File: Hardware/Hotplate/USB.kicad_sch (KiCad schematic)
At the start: 14 parts, among them IC2 FT231XQ-T, J8 GSB1C41110SSHR

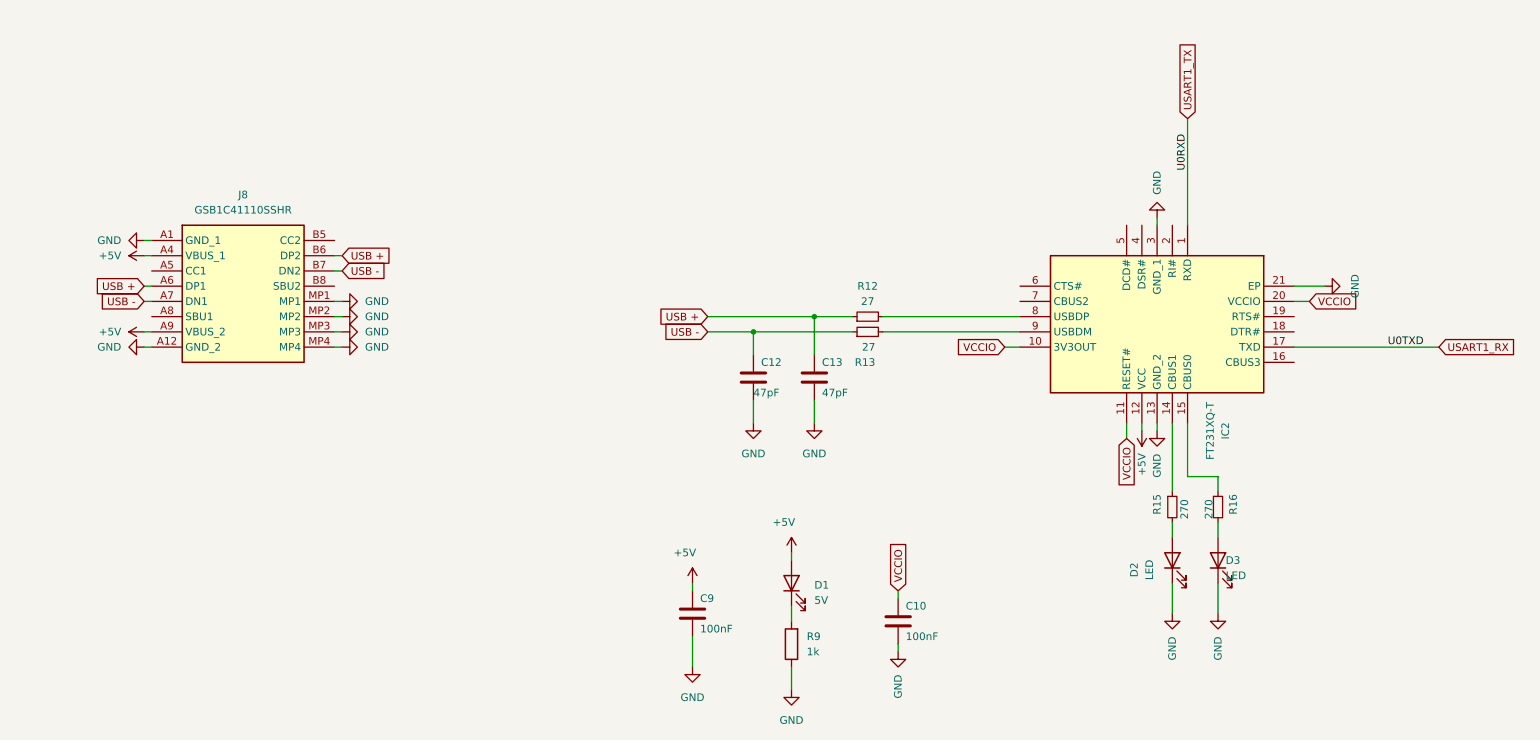
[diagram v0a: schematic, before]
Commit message: V2
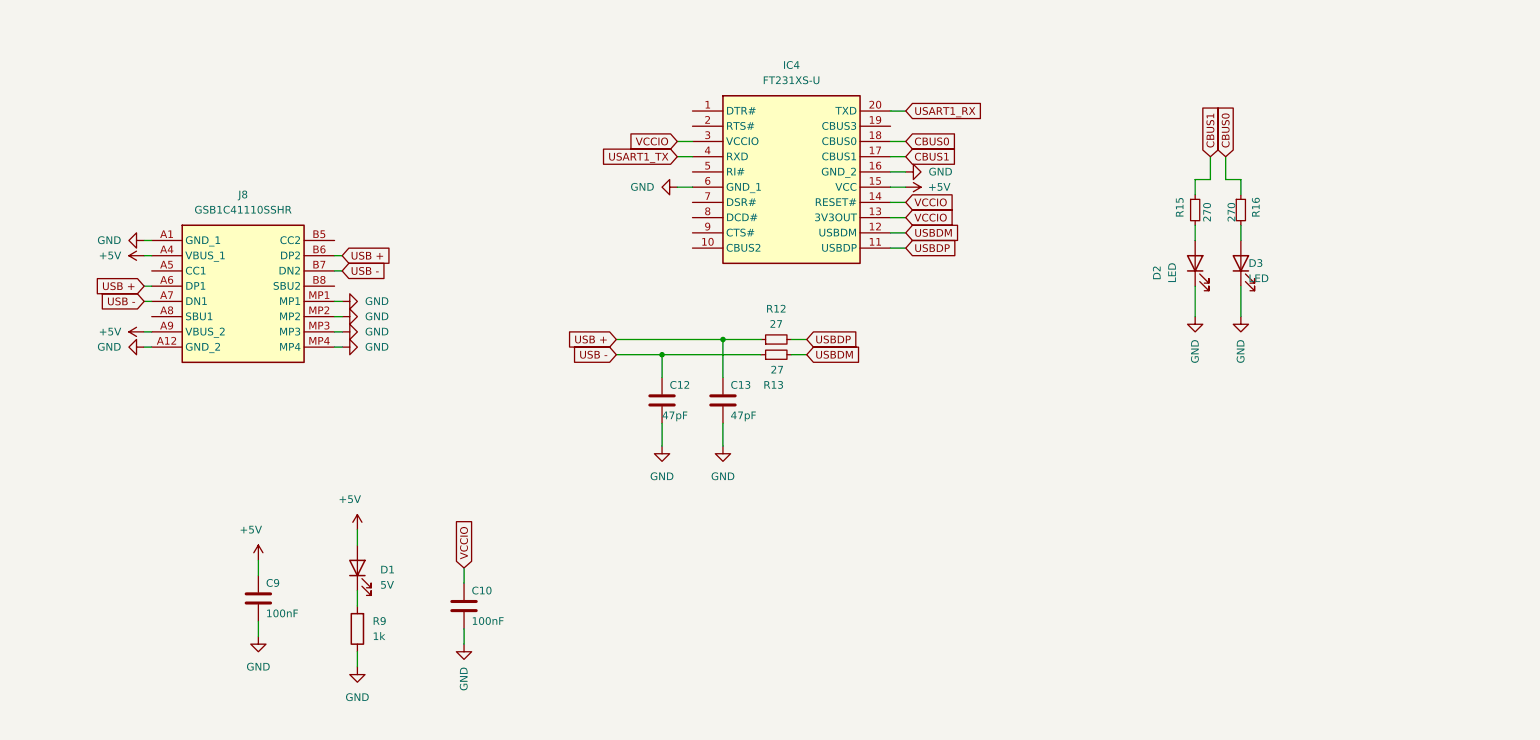
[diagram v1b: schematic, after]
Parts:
- removed IC2: FT231XQ-T, QFN50P400X400X80-21N, symbol SamacSys_Parts:FT231XQ-T
- added IC4: FT231XS-U, SOP64P599X175-20N, symbol SamacSys_Parts:FT231XS-U
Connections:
- net +5V: now also IC4.15 (VCC)
- net GND: now also IC4.16 (GND_2), IC4.6 (GND_1)
- net USART1_RX: now also IC4.20 (TXD)
- net USART1_TX: now also IC4.4 (RXD)
- net VCCIO: now also IC4.13 (3V3OUT), IC4.14 (RESET#), IC4.3 (VCCIO)
- net CBUS1: now reaches R15.1
- net CBUS1: now also IC4.17 (CBUS1)
- net CBUS0: now reaches R16.1
- net CBUS0: now also IC4.18 (CBUS0)
- net USBDM: now reaches R13.2
- net USBDM: now also IC4.12 (USBDM)
- net USBDP: now reaches R12.2
- net USBDP: now also IC4.11 (USBDP)
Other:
- moved on the sheet: C10, C12, C13, C9, D1, D2, D3, R12, R13, R15, R16, R9

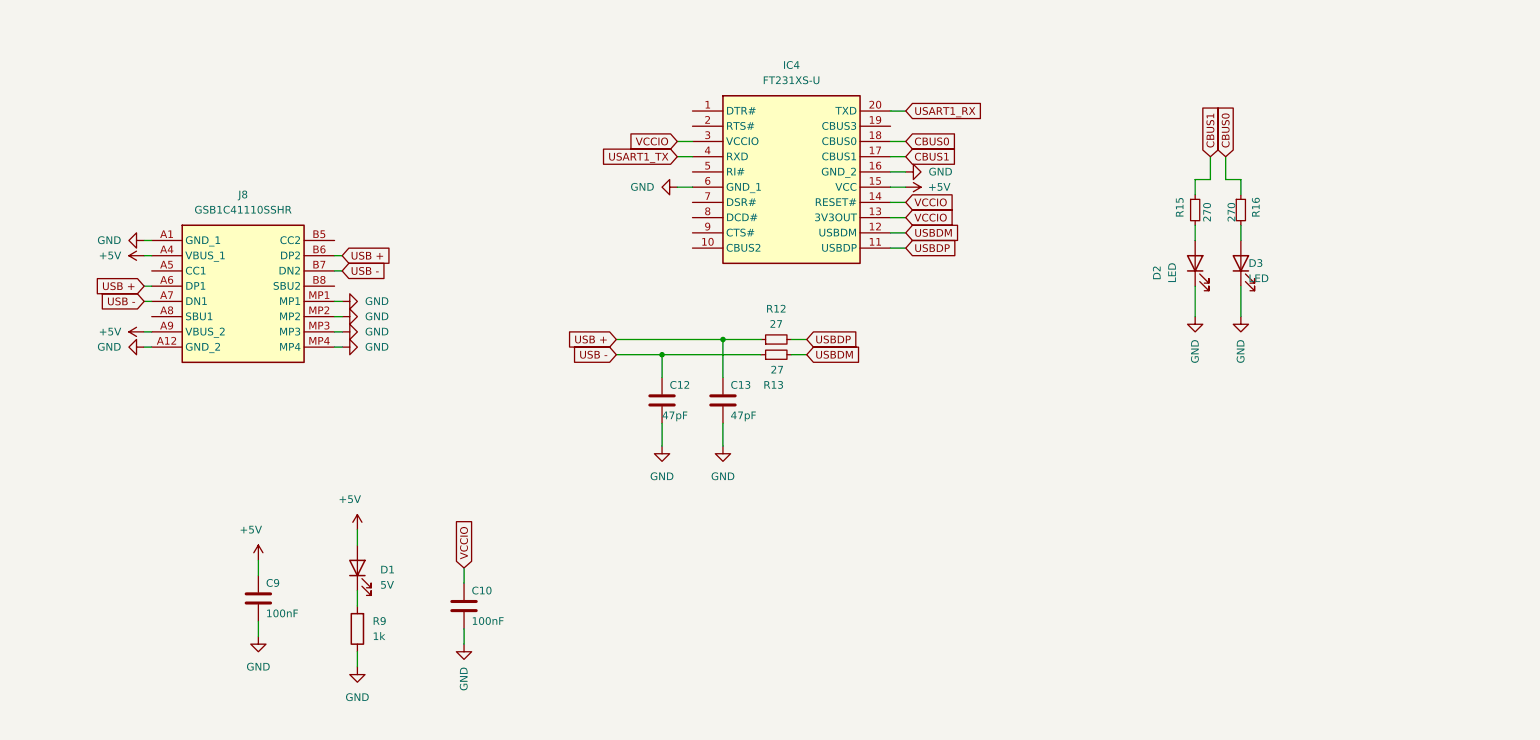
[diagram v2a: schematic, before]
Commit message: made it pretty (#8)
Co-authored-by: nexophoenixe <jan.gradwohl2005@mail.com>
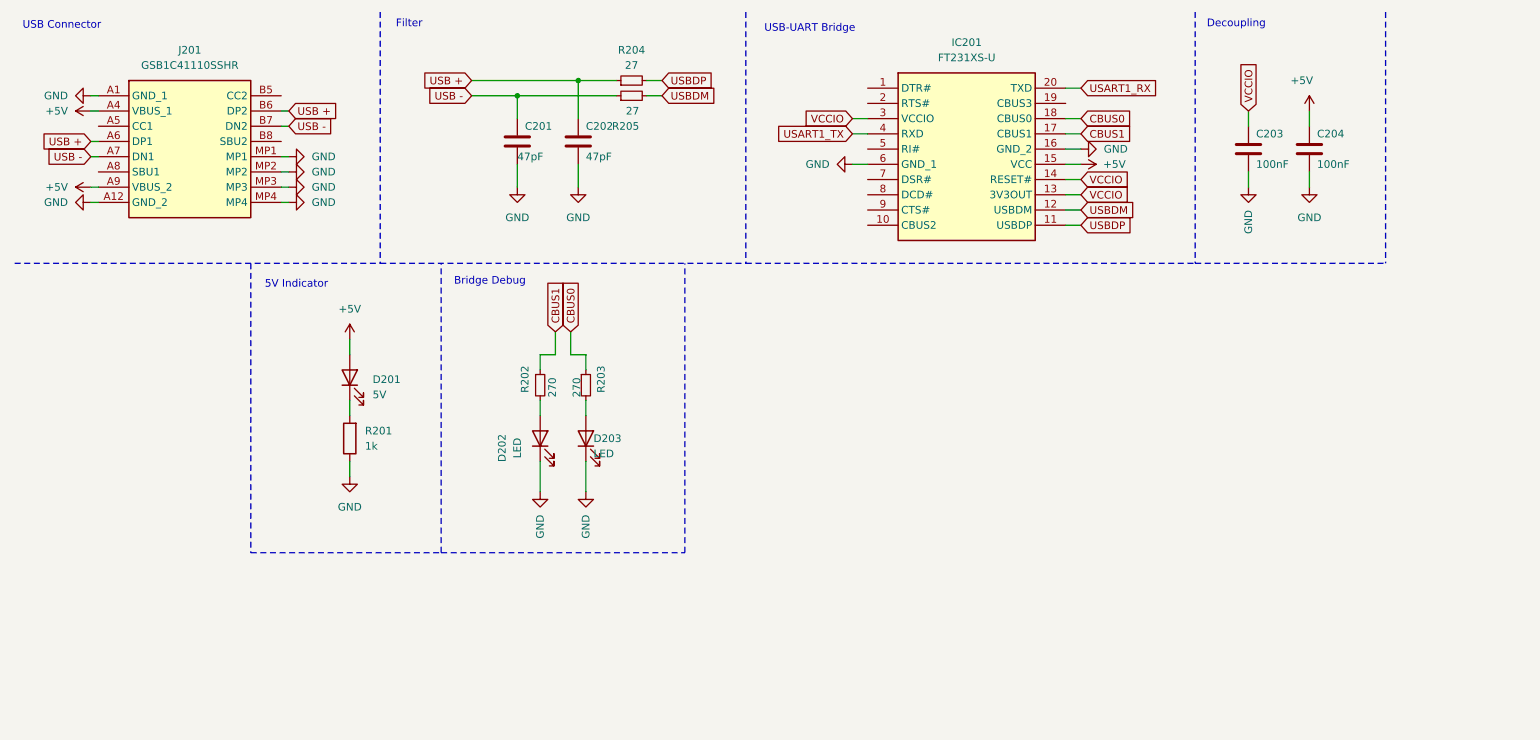
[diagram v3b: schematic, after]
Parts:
- renumbered C12 to C201, C13 to C202, C10 to C203, C9 to C204, D1 to D201, D2 to D202, D3 to D203, IC4 to IC201, J8 to J201, R9 to R201, R15 to R202, R16 to R203, R12 to R204, R13 to R205
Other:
- note added: "5V Indicator"
- note added: "Bridge Debug"
- note added: "Decoupling"
- note added: "Filter"
- note added: "USB Connector"
- note added: "USB-UART Bridge"
- moved on the sheet: C201, C202, C203, C204, D201, D202, D203, IC201, J201, R201, R202, R203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
